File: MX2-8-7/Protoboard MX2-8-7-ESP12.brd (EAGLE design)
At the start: 64.4 x 71.2 mm, 145 parts, among them X1 ESP-12E

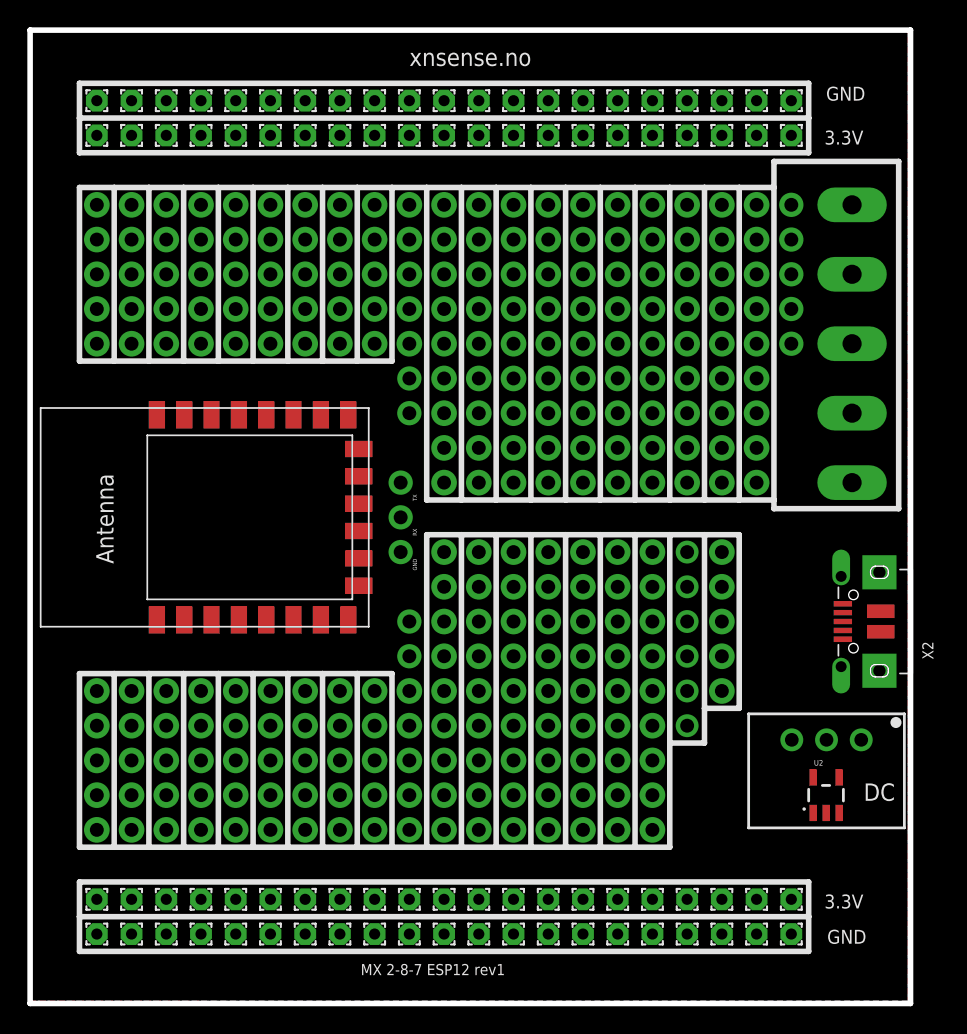
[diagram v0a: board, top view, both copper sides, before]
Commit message: Routed
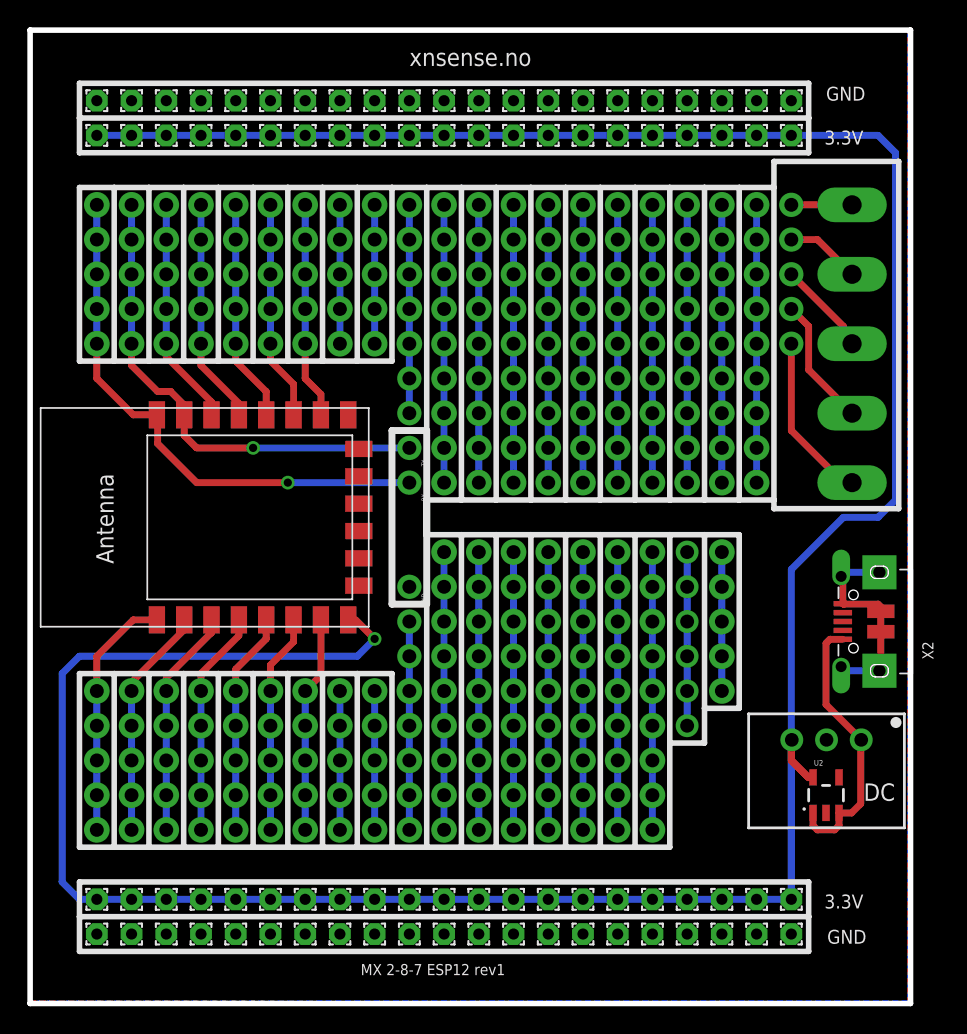
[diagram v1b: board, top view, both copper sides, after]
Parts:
- moved J8 15.2 mm to (5.08, 48.3)
- moved J7 10.2 mm to (7.62, 48.3)
- moved J4 5.08 mm to (17.8, 48.3)
- moved J3 5.08 mm to (15.2, 48.3)
- moved J39 5.08 mm to (10.2, 48.3)
- moved J5 5.08 mm to (20.3, 48.3)
- moved J2 5.08 mm to (12.7, 48.3)
- moved GND 2.62 mm to (27.9, 30.5)
- moved RX 2.62 mm to (27.9, 38.1)
- moved TX 2.62 mm to (27.9, 40.6)
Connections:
- removed net N$7: J7.1, J7.2, J7.3, J7.4, J7.5
- removed net N$8: J8.1, J8.2, J8.3, J8.4, J8.5
- net N$45: now also J7.1, J7.2, J7.3, J7.4, J7.5
- net N$46: now also J8.1, J8.2, J8.3, J8.4, J8.5
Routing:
- net VDD: track 0.00 -> 229.0 mm, vias 0 -> 1
- net N$46: track 0.00 -> 39.9 mm, vias 0 -> 1
- net N$45: track 0.00 -> 35.9 mm, vias 0 -> 1
- net N$39: track 0.00 -> 20.3 mm
- net N$38: track 0.00 -> 20.3 mm
- net N$37: track 0.00 -> 20.3 mm
- net N$36: track 0.00 -> 20.3 mm
- net N$35: track 0.00 -> 20.3 mm
- net N$33: track 0.00 -> 20.3 mm
- net N$32: track 0.00 -> 20.3 mm
- net N$21: track 0.00 -> 20.3 mm
- net N$20: track 0.00 -> 20.3 mm
- net N$19: track 0.00 -> 20.3 mm
- net N$18: track 0.00 -> 20.3 mm
- net N$17: track 0.00 -> 20.3 mm
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
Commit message: Revert "Routed"
This reverts commit 078e80659a45ef39a7709107a01737087c5908e1.
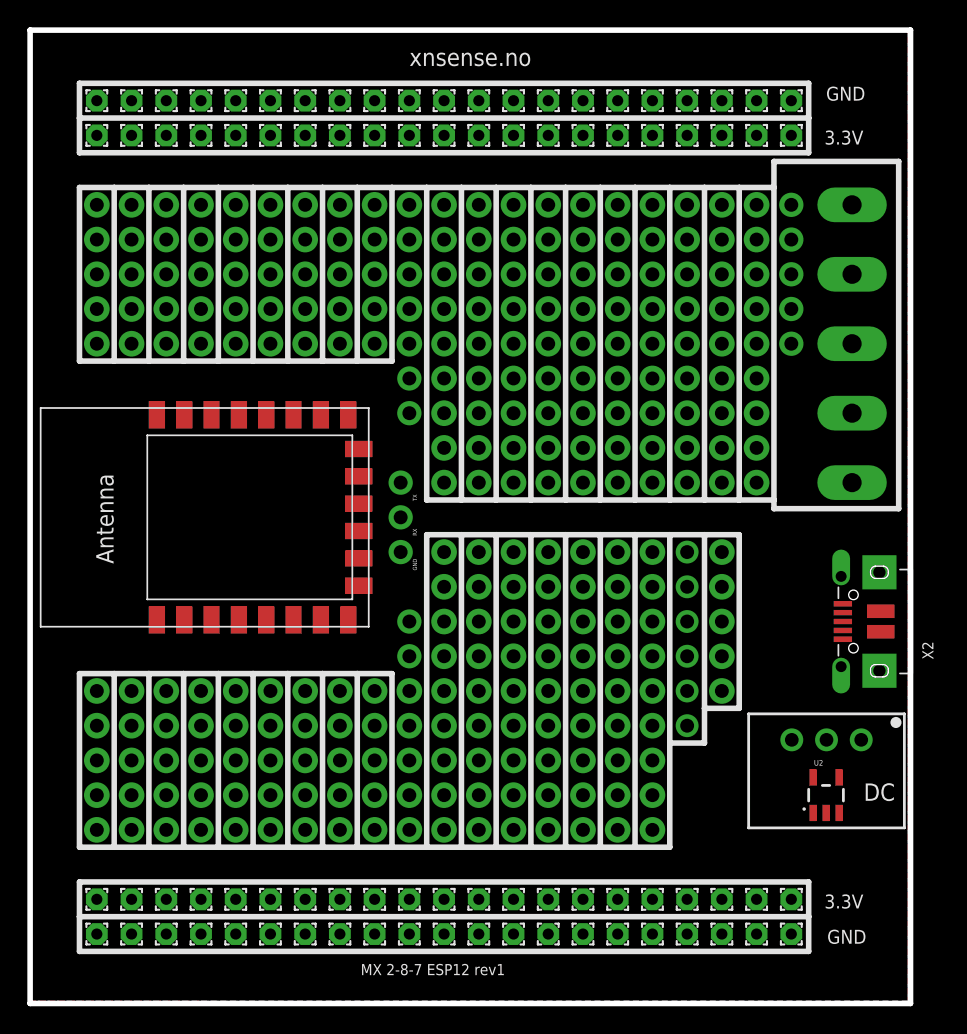
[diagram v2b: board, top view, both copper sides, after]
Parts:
- moved J8 15.2 mm to (20.3, 48.3)
- moved J7 10.2 mm to (17.8, 48.3)
- moved J4 5.08 mm to (12.7, 48.3)
- moved J3 5.08 mm to (10.2, 48.3)
- moved J39 5.08 mm to (5.08, 48.3)
- moved J5 5.08 mm to (15.2, 48.3)
- moved J2 5.08 mm to (7.62, 48.3)
- moved GND 2.62 mm to (27.3, 33.0)
- moved RX 2.62 mm to (27.3, 35.6)
- moved TX 2.62 mm to (27.3, 38.1)
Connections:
- new net N$7: J7.1, J7.2, J7.3, J7.4, J7.5
- new net N$8: J8.1, J8.2, J8.3, J8.4, J8.5
- net N$45: no longer J7.1, J7.2, J7.3, J7.4, J7.5
- net N$46: no longer J8.1, J8.2, J8.3, J8.4, J8.5
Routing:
- net VDD: track 229.0 -> 0.00 mm, vias 1 -> 0
- net N$46: track 39.9 -> 0.00 mm, vias 1 -> 0
- net N$45: track 35.9 -> 0.00 mm, vias 1 -> 0
- net N$39: track 20.3 -> 0.00 mm
- net N$38: track 20.3 -> 0.00 mm
- net N$37: track 20.3 -> 0.00 mm
- net N$36: track 20.3 -> 0.00 mm
- net N$35: track 20.3 -> 0.00 mm
- net N$33: track 20.3 -> 0.00 mm
- net N$32: track 20.3 -> 0.00 mm
- net N$21: track 20.3 -> 0.00 mm
- net N$20: track 20.3 -> 0.00 mm
- net N$19: track 20.3 -> 0.00 mm
- net N$18: track 20.3 -> 0.00 mm
- net N$17: track 20.3 -> 0.00 mm
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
